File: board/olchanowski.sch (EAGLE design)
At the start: 202 parts, among them IC1 LPC1768, J1 X-AXIS, J10 B4B-XH-A(LF)(SN), J2 Y-AXIS, J3 Z_AXIS, J4 ARJM11D7-009-AB-ER2-T, J5 RGB LED, J6 USB-C-FEMALE, J7 1744428-4, J8 282814-4, J9 1-281742-2, P1 TPSM53602, Q1 12MHz, Q10 SSM3K329R,LF, Q11 SSM3K329R,LF, Q2 25MHz, Q3 SIJA58DP, Q4 SIJA58DP, Q5 SSM3K329R,LF, Q6 SSM3K329R,LF, Q7 SSM3K329R,LF, Q8 SSM3K329R,LF, Q9 PFETSM, SW1 SPST-2-4PIN, SW2 SPST-2-4PIN, U1 TMC2209-LA, U2 TMC2209-LA, U3 TMC2209-LA, U4 TMC2209-LA, U5 LAN8720, U6 74HC1G04, U7 LM5111, U8 NCP5661-0, U9 PCA9306DCTR, X1 X-AXIS, X2 Y-AXIS, X3 Z-AXIS, X4 FAN, X5 LCD, X6 HB THERM, X7 SENSER

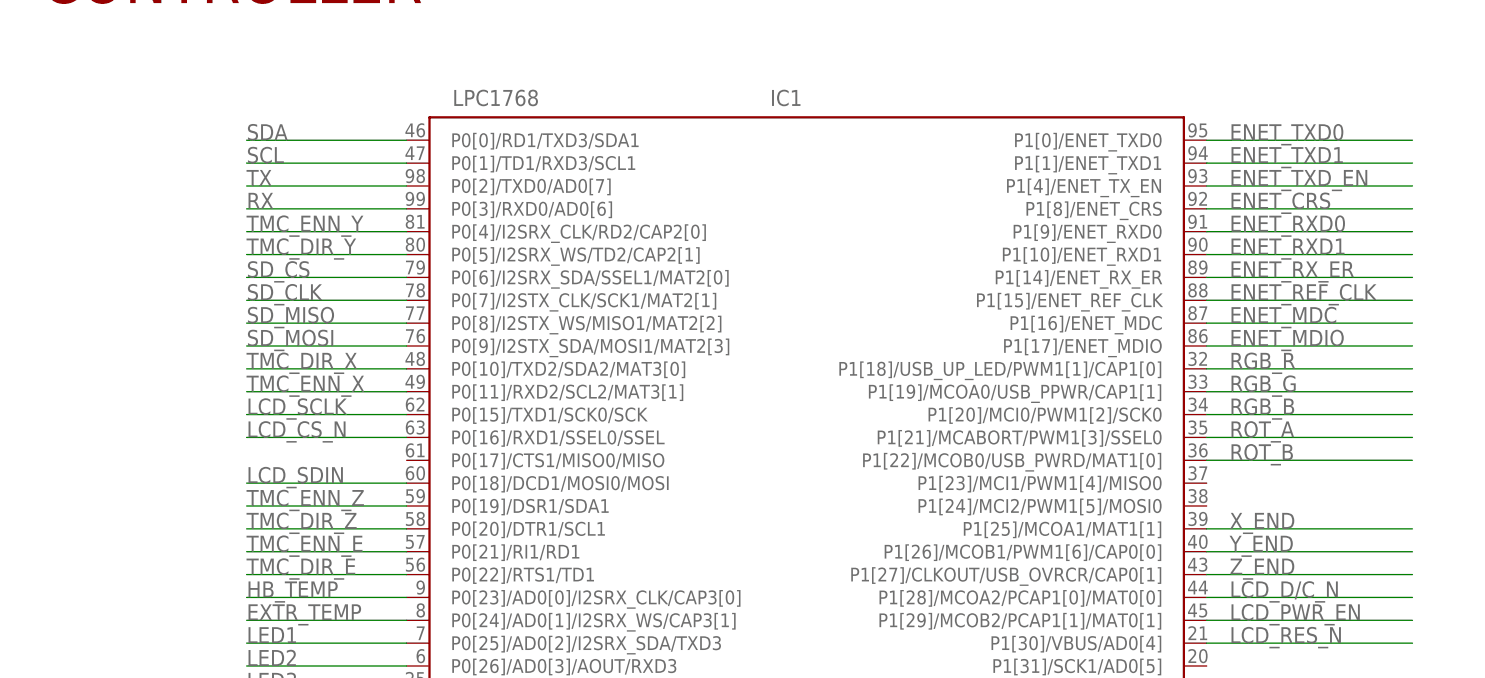
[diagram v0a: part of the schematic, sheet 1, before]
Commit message: First rev done and ordered!
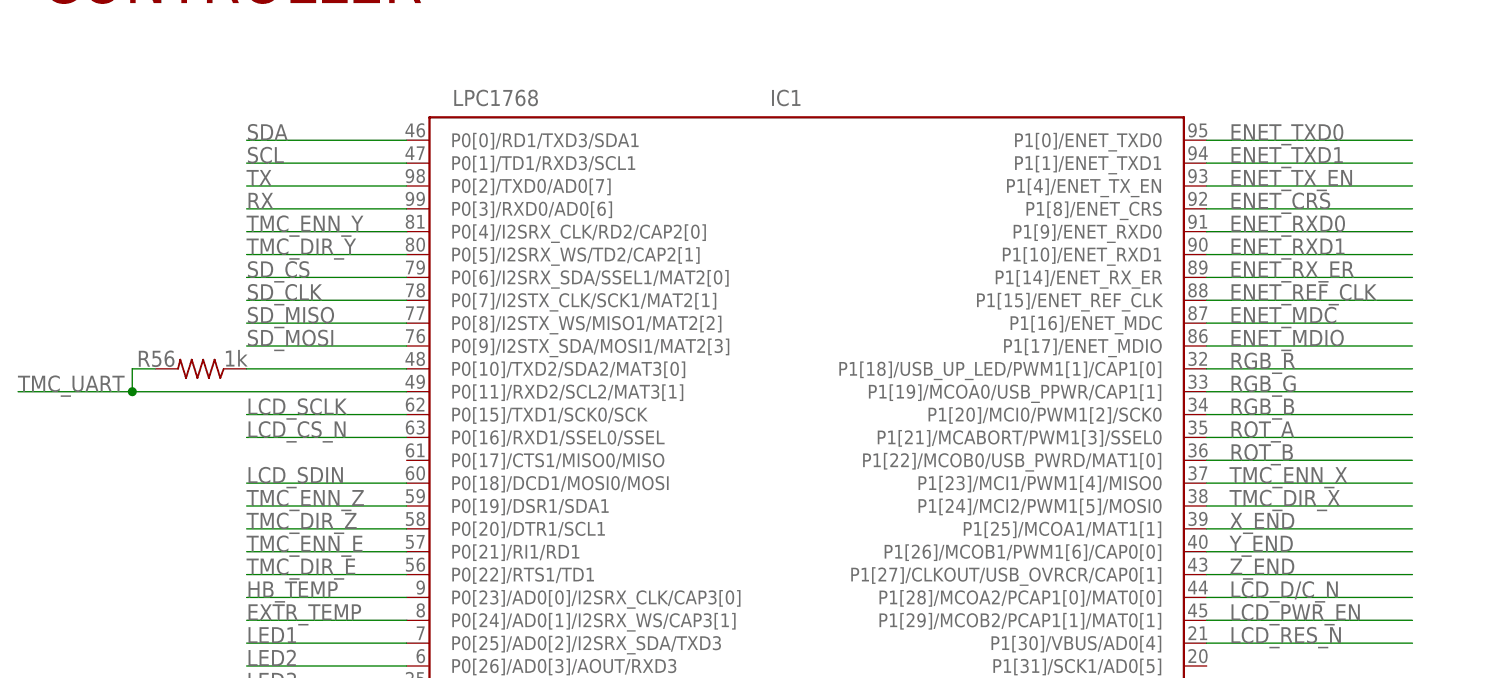
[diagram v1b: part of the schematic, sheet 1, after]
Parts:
- added R56: (no value), rcl:R-US_R0402
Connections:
- removed net ENET_TXD_EN: IC1.P1[4]/ENET_TX_EN
- new net N$47: IC1.P0[10]/TXD2/SDA2/MAT3[0], R56.1
- net ENET_TX_EN: now also IC1.P1[4]/ENET_TX_EN
- net TMC_DIR_X: now also IC1.P1[24]/MCI2/PWM1[5]/MOSI0; no longer IC1.P0[10]/TXD2/SDA2/MAT3[0]
- net TMC_ENN_X: now also IC1.P1[23]/MCI1/PWM1[4]/MISO0; no longer IC1.P0[11]/RXD2/SCL2/MAT3[1]
- net TMC_UART: now also IC1.P0[11]/RXD2/SCL2/MAT3[1], R56.2
